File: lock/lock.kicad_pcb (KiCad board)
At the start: 2 copper layers, 92.1 x 58 mm, 7 parts, among them J1 Screw_Terminal_01x02

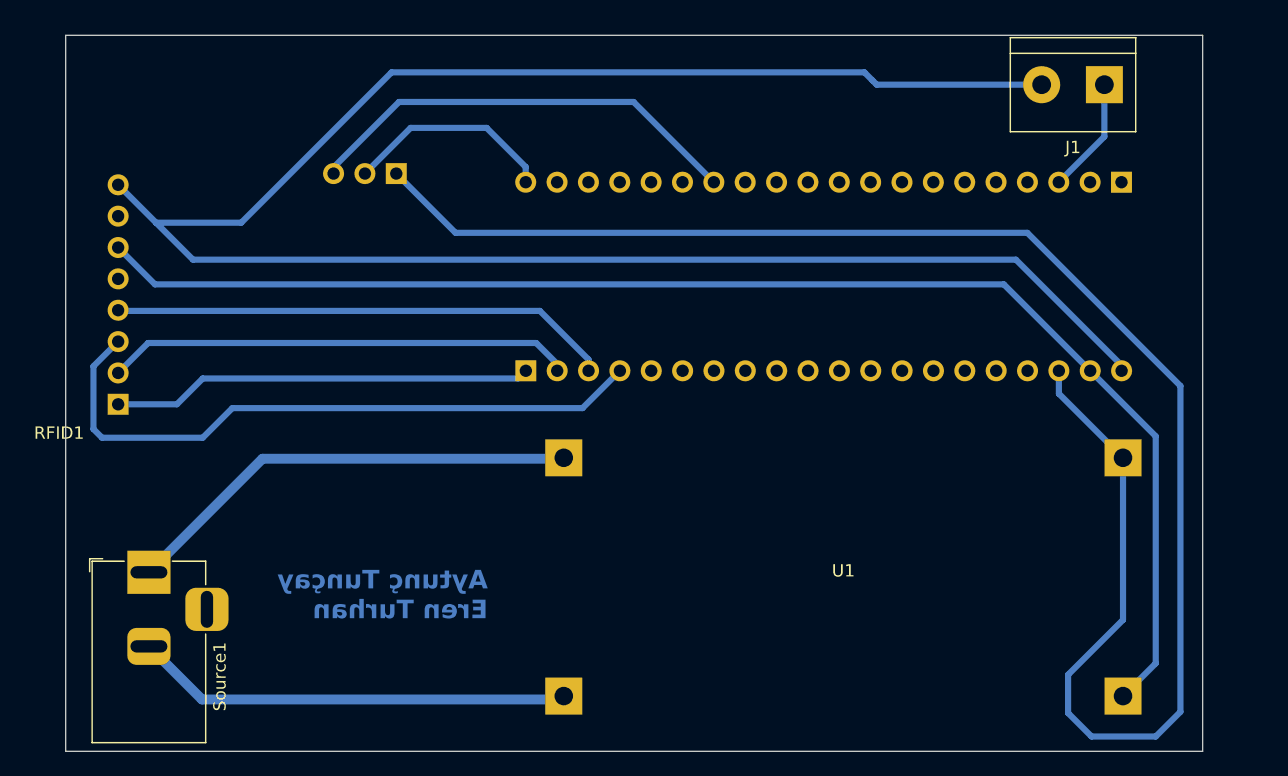
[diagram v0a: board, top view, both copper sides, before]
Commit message: Final
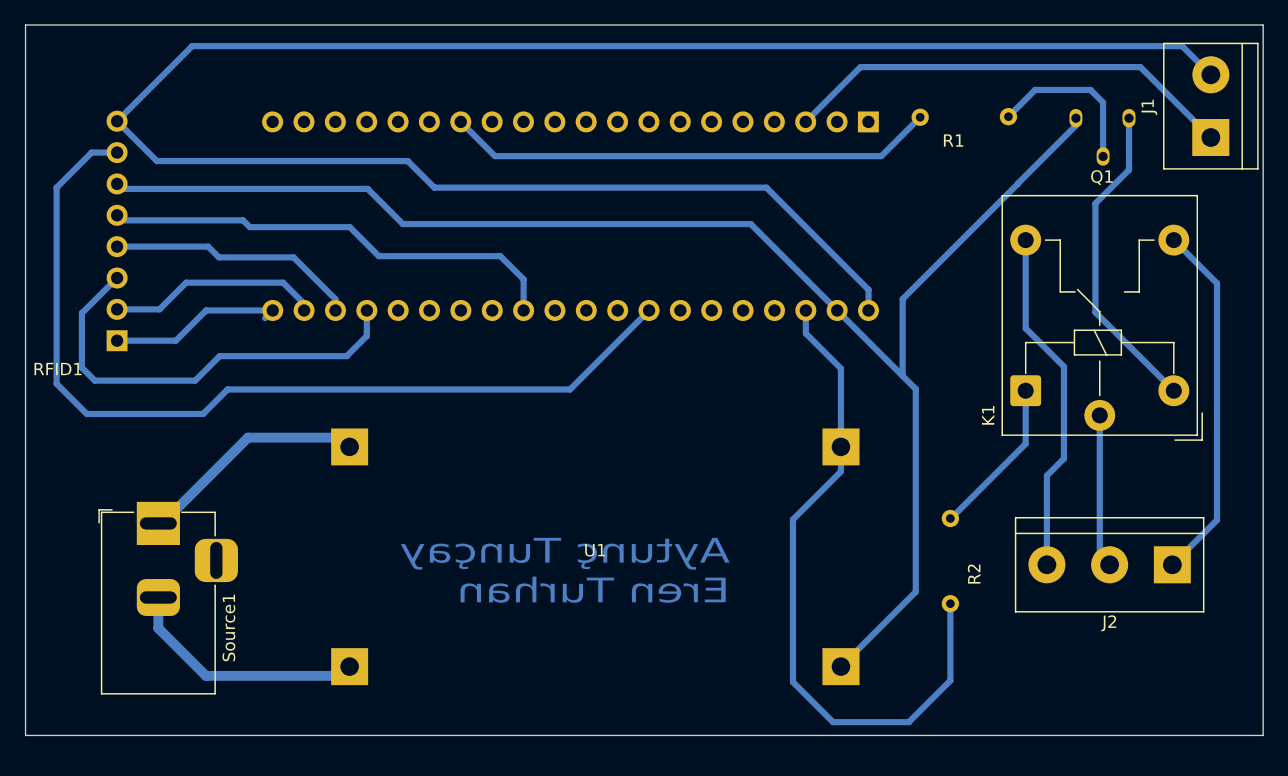
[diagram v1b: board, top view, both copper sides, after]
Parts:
- removed Relay2: Relay IN, Connector_PinHeader_2.54mm:PinHeader_1x03_P2.54mm_Horizontal
- added J2: Screw_Terminal_01x03, TerminalBlock:TerminalBlock_bornier-3_P5.08mm, F.Cu at (185.4, 116.0)
- added K1: JQC-3FF-005-1Z, Relay_THT:Relay_SPDT_Hongfa_JQC-3FF_0XX-1Z, F.Cu at (173.6, 101.9)
- added Q1: BC547, Package_TO_SOT_THT:TO-92_Inline, F.Cu at (181.0, 81.0)
- added R1: R, Resistor_THT:R_Axial_DIN0204_L3.6mm_D1.6mm_P1.90mm_Vertical, F.Cu at (168.7, 79.7)
- added R2: R, Resistor_THT:R_Axial_DIN0204_L3.6mm_D1.6mm_P1.90mm_Vertical, F.Cu at (167.5, 115.8)
- moved STM1 21.1 mm to (112.6, 95.4)
- moved STM2 21.1 mm to (160.8, 80.1)
- moved U1 20.2 mm to (138.7, 115.3)
- moved J1 9.63 mm to (188.6, 81.4), turned to 90 degrees
- moved RFID1 5.15 mm to (99.5, 97.9)
- moved Source1 4.03 mm to (103.3, 112.6)
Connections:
- net Net-(J1-Pin_2) renamed +3V3
- net Net-(RFID1-Pin_1) renamed SS
- net Net-(RFID1-Pin_2) renamed SCK
- net Net-(RFID1-Pin_3) renamed MOSI
- net Net-(RFID1-Pin_4) renamed MISO
- net Net-(Relay2-Pin_1) renamed +5V
- net Normally Closed renamed +12V
- RFID1 pad 5: unconnected-(RFID1-Pin_5-Pad5) -> RST
- RFID1 pad 6: Net-(RFID1-Pin_6) -> GND
- RFID1 pad 7: unconnected-(RFID1-Pin_7-Pad7) -> INT
- STM1 pad 13: unconnected-(STM1-Pin_13-Pad13) -> INT
- STM1 pad 19: Net-(RFID1-Pin_6) -> GND
- STM1 pad 9: unconnected-(STM1-Pin_9-Pad9) -> RST
- STM2 pad 14: Net-(Relay2-Pin_3) -> relayControl
- STM2 pad 20: Net-(Relay2-Pin_2) -> unconnected-(STM2-Pin_20-Pad20)
- Source1 pad 2: Lock Output -> GND
- U1 pad 2: Lock Output -> GND
- U1 pad 4: Net-(RFID1-Pin_6) -> GND
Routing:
- net GND: track 0.00 -> 143.2 mm
- net Net-(RFID1-Pin_6): track 112.5 -> 0.00 mm
- net +5V: track 139.5 -> 54.6 mm
- net INT: track 0.00 -> 74.4 mm
- net relayControl: track 0.00 -> 39.7 mm
- net RST: track 0.00 -> 37.6 mm
- net Net-(Relay2-Pin_3): track 36.2 -> 0.00 mm
- net Lock Output: track 36.1 -> 0.00 mm
- net Net-(J2-Pin_1): track 0.00 -> 29.2 mm
- net Net-(J2-Pin_3): track 0.00 -> 28.2 mm
- net Net-(J1-Pin_1): track 9.43 -> 37.0 mm
- net Net-(Q1-C): track 0.00 -> 25.8 mm
- net SCK: track 37.8 -> 17.3 mm
- net MISO: track 40.7 -> 20.4 mm
- net SS: track 34.1 -> 14.5 mm
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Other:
- board size 92.1 x 58 mm -> 100.2 x 57.5 mm
